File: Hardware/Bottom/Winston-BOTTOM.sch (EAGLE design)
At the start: 32 parts, among them U1 AD5242-SO16

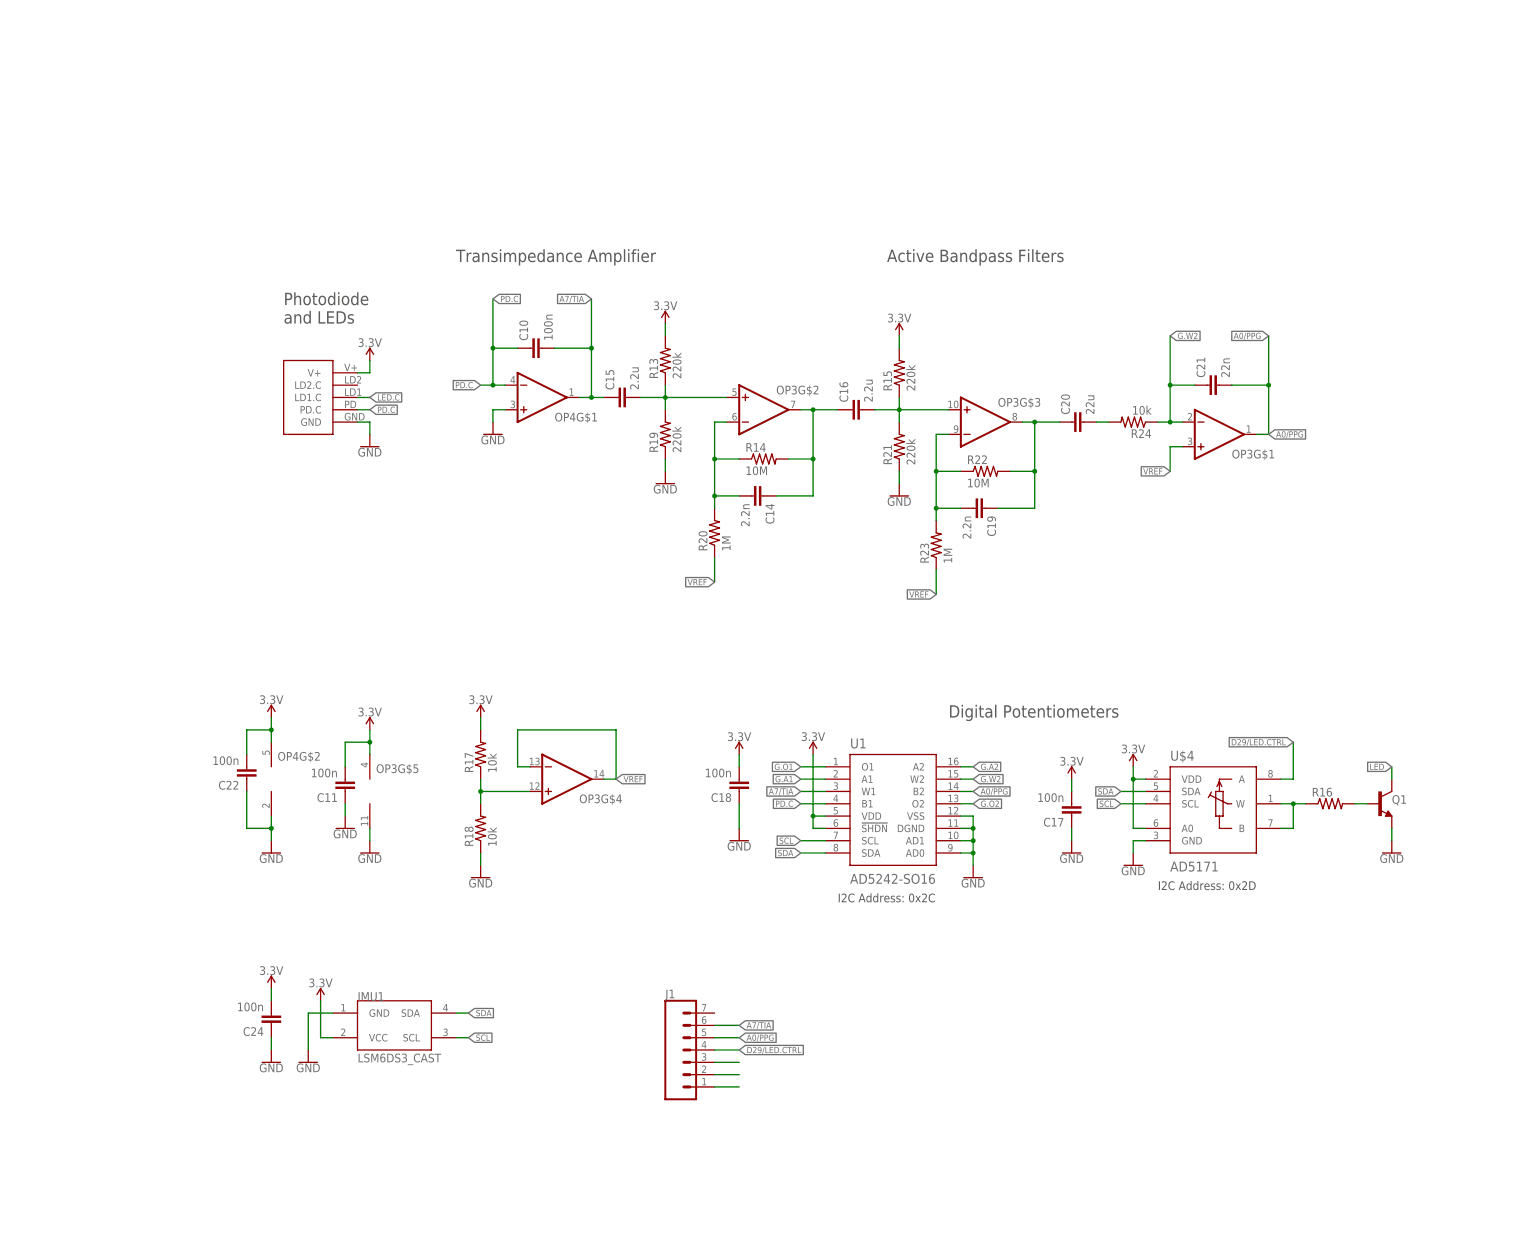
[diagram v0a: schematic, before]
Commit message: finished routing all boards
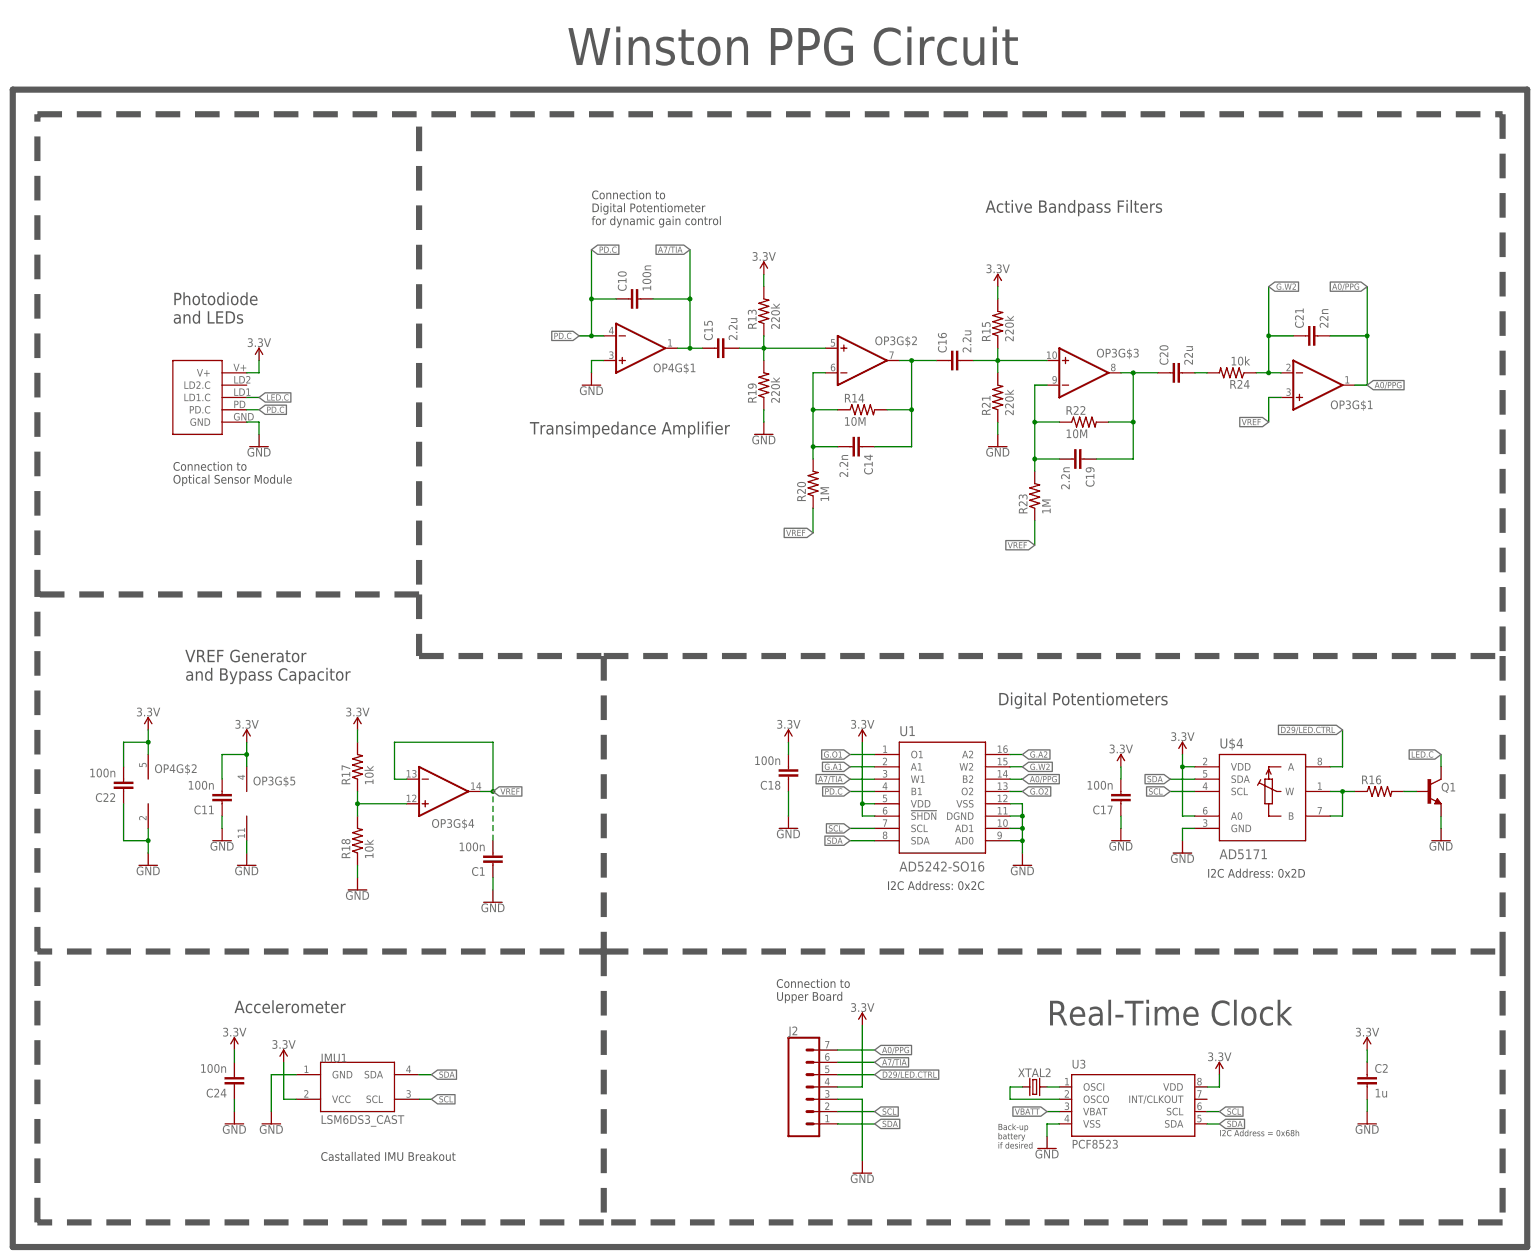
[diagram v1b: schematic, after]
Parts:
- removed J1: (no value), LinnesLab-Connectors:CONN_07
- added C1: 100n, LinnesLab-Passives:CAPACITOR0603
- added C2: 1u, LinnesLab-Passives:CAPACITOR0603
- added J2: (no value), LinnesLab-Connectors:CONN_07-1.27MM
- added U3: PCF8523, LinnesLab-Clocks:PCF8523
- added XTAL2: 32.7680kHz, LinnesLab-Clocks:CRYSTALECS-.327-12.5-12-C-TR
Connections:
- removed net LED: Q1.C
- removed net N$11: J1.1
- removed net N$6: J1.3
- removed net N$7: J1.2
- new net N$1: U3.OSCO, XTAL2.1
- new net N$2: U3.OSCI, XTAL2.2
- new net VBATT: U3.VBAT
- net 3.3V: now also C2.1, J2.4, U3.VDD
- net A0/PPG: now also J2.7; no longer J1.5
- net A7/TIA: now also J2.6; no longer J1.6
- net D29/LED.CTRL: now also J2.5; no longer J1.4
- net GND: now also C1.1, C2.2, J2.3, U3.VSS
- net LED.C: now also Q1.C
- net SCL: now also J2.2, U3.SCL
- net SDA: now also J2.1, U3.SDA
- net VREF: now also C1.2
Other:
- note added: "Accelerometer"
- note added: "Back-up battery if desired"
- note added: "Castallated IMU Breakout"
- note added: "Connection to Digital Potentiometer for dynamic gain control"
- note added: "Connection to Optical Sensor Module"
- note added: "Connection to Upper Board"
- note added: "I2C Address = 0x68h"
- note added: "Real-Time Clock"
- note added: "VREF Generator and Bypass Capacitor"
- note added: "Winston PPG Circuit"
- moved on the sheet: C10, C11, C14, C15, C16, C17, C18, C19, C20, C21, C22, C24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
